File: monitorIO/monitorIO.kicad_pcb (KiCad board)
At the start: 2 copper layers, 9.1 x 23.3 mm, 17 parts, among them J1 Conn_01x09_Female

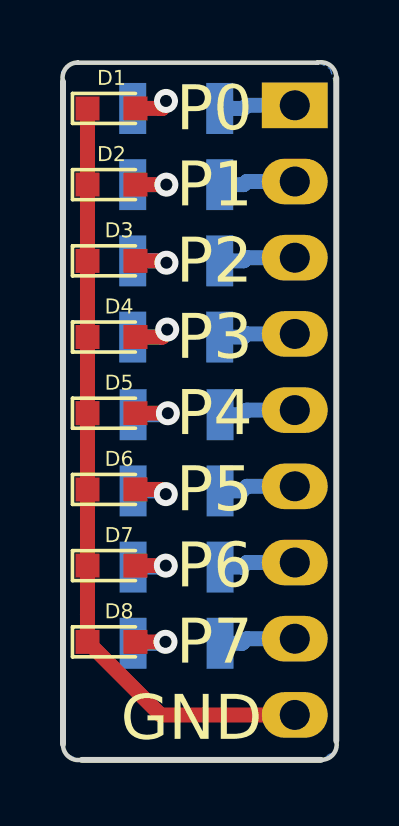
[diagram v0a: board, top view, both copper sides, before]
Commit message: changes in monitor led
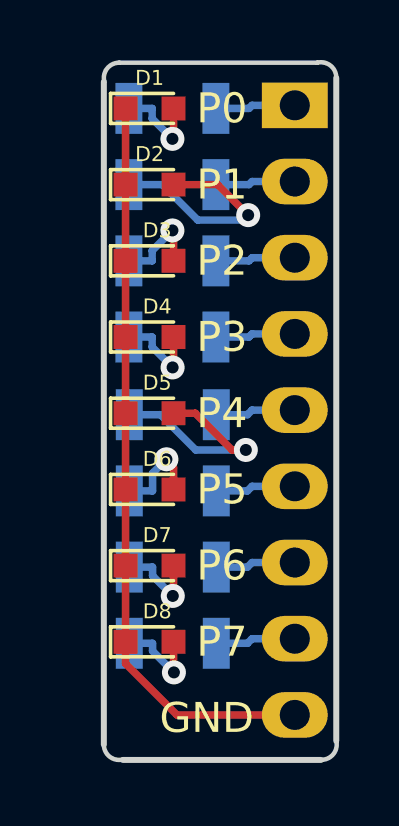
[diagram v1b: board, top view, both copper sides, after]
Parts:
- moved D1 1.27 mm to (141.9, 78.7)
- moved D2 1.27 mm to (141.9, 81.3)
- moved D3 1.27 mm to (141.9, 83.8)
- moved D4 1.27 mm to (141.9, 86.4)
- moved D5 1.27 mm to (141.9, 88.9)
- moved D6 1.27 mm to (141.9, 91.4)
- moved D7 1.27 mm to (141.9, 94.0)
- moved D8 1.27 mm to (141.9, 96.5)
- moved R1 0.13 mm to (142.6, 78.7)
- moved R2 0.13 mm to (142.6, 81.3)
- moved R3 0.13 mm to (142.6, 83.8)
- moved R4 0.13 mm to (142.6, 86.4)
- moved R5 0.13 mm to (142.6, 88.9)
- moved R6 0.13 mm to (142.6, 91.5)
- moved R7 0.13 mm to (142.6, 94.0)
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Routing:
- net Net-(D2-Pad2): track 2.15 -> 7.44 mm
- net Net-(D5-Pad2): track 2.26 -> 7.29 mm
- net Net-(D8-Pad2): track 2.10 -> 3.06 mm
- net Net-(D7-Pad2): track 2.12 -> 3.04 mm
- net Net-(D6-Pad2): track 2.24 -> 3.12 mm
- net Net-(D3-Pad2): track 2.21 -> 3.10 mm
- net GND: track 25.7 -> 24.9 mm
- net Net-(D1-Pad2): track 2.46 -> 3.10 mm
- net Net-(D4-Pad2): track 2.50 -> 3.10 mm
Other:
- board size 9.1 x 23.3 mm -> 7.8 x 23.3 mm
- net class Default: trace_width 0.5 -> 0.25
- board text added: "WhatsApp 6677983021"
- board text added: "abeleduardo.hdz@gmail.com"
